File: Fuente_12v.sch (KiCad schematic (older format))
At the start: 3 parts, among them U1 L7812

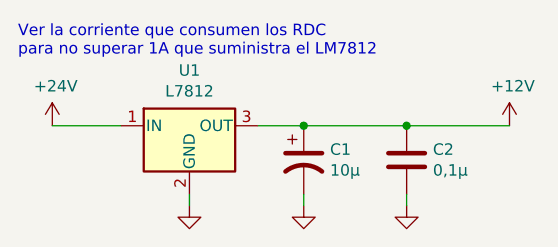
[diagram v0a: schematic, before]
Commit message: cambios en el placement
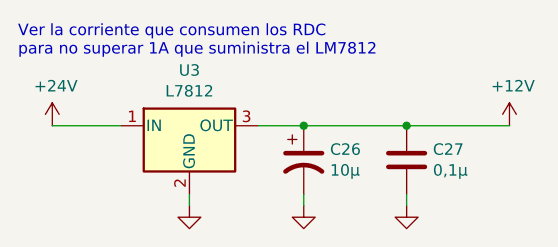
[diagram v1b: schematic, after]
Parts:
- renumbered C1 to C26, C2 to C27, U1 to U3
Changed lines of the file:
@@
 P 3100 2100
 AR Path="/5EF448F6" Ref="U?"  Part="1"
-AR Path="/5EF34214/5EF448F6" Ref="U1"  Part="1"
-F 0 "U1" H 3100 2342 50  0000 C CNN
+AR Path="/5EF34214/5EF448F6" Ref="U3"  Part="1"
+F 0 "U3" H 3100 2342 50  0000 C CNN
 F 1 "L7812" H 3100 2251 50  0000 C CNN
 F 2 "Package_TO_SOT_THT:TO-218-3_Vertical" H 3125 1950 50  0001 L CIN
@@
 P 3100 2450
 AR Path="/5EF44904" Ref="#PWR?"  Part="1"
-AR Path="/5EF34214/5EF44904" Ref="#PWR0102"  Part="1"
-F 0 "#PWR0102" H 3100 2450 30  0001 C CNN
+AR Path="/5EF34214/5EF44904" Ref="#PWR046"  Part="1"
+F 0 "#PWR046" H 3100 2450 30  0001 C CNN
 F 1 "GND" H 3100 2380 30  0001 C CNN
 F 2 "" H 3100 2450 60  0000 C CNN
@@
 P 3600 2450
 AR Path="/5EF4490B" Ref="#PWR?"  Part="1"
-AR Path="/5EF34214/5EF4490B" Ref="#PWR0103"  Part="1"
-F 0 "#PWR0103" H 3600 2450 30  0001 C CNN
+AR Path="/5EF34214/5EF4490B" Ref="#PWR047"  Part="1"
+F 0 "#PWR047" H 3600 2450 30  0001 C CNN
 F 1 "GND" H 3600 2380 30  0001 C CNN
 F 2 "" H 3600 2450 60  0000 C CNN
@@
 P 4050 2250
 AR Path="/5EF44912" Ref="C?"  Part="1"
-AR Path="/5EF34214/5EF44912" Ref="C2"  Part="1"
-F 0 "C2" H 4165 2296 50  0000 L CNN
+AR Path="/5EF34214/5EF44912" Ref="C27"  Part="1"
+F 0 "C27" H 4165 2296 50  0000 L CNN
 F 1 "0,1µ" H 4165 2205 50  0000 L CNN
 F 2 "Capacitor_SMD:C_1206_3216Metric_Pad1.42x1.75mm_HandSolder" H 4088 2100 50  0001 C CNN
@@
 P 4050 2450
 AR Path="/5EF44918" Ref="#PWR?"  Part="1"
-AR Path="/5EF34214/5EF44918" Ref="#PWR0104"  Part="1"
-F 0 "#PWR0104" H 4050 2450 30  0001 C CNN
+AR Path="/5EF34214/5EF44918" Ref="#PWR048"  Part="1"
+F 0 "#PWR048" H 4050 2450 30  0001 C CNN
 F 1 "GND" H 4050 2380 30  0001 C CNN
 F 2 "" H 4050 2450 60  0000 C CNN
@@
 P 4500 2100
 AR Path="/5EF44921" Ref="#PWR?"  Part="1"
-AR Path="/5EF34214/5EF44921" Ref="#PWR0105"  Part="1"
-F 0 "#PWR0105" H 4500 1950 50  0001 C CNN
+AR Path="/5EF34214/5EF44921" Ref="#PWR045"  Part="1"
+F 0 "#PWR045" H 4500 1950 50  0001 C CNN
 F 1 "+12V" H 4515 2273 50  0000 C CNN
 F 2 "" H 4500 2100 50  0001 C CNN
@@
 P 2500 2100
 AR Path="/5EF448F0" Ref="#PWR?"  Part="1"
-AR Path="/5EF34214/5EF448F0" Ref="#PWR0101"  Part="1"
-F 0 "#PWR0101" H 2500 1950 50  0001 C CNN
+AR Path="/5EF34214/5EF448F0" Ref="#PWR044"  Part="1"
+F 0 "#PWR044" H 2500 1950 50  0001 C CNN
 F 1 "+24V" H 2515 2273 50  0000 C CNN
 F 2 "" H 2500 2100 50  0001 C CNN
@@
 	2500 2100 2800 2100
 $Comp
-L Device:CP1 C1
+L Device:CP1 C26
 U 1 1 5F0A8BCC
 P 3600 2250
-F 0 "C1" H 3715 2296 50  0000 L CNN
+F 0 "C26" H 3715 2296 50  0000 L CNN
 F 1 "10µ" H 3715 2205 50  0000 L CNN
 F 2 "Capacitor_SMD:CP_Elec_4x5.4" H 3600 2250 50  0001 C CNN
